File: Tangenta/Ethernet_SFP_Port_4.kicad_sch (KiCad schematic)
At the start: 17 parts, among them J9 HC-SFP-01L

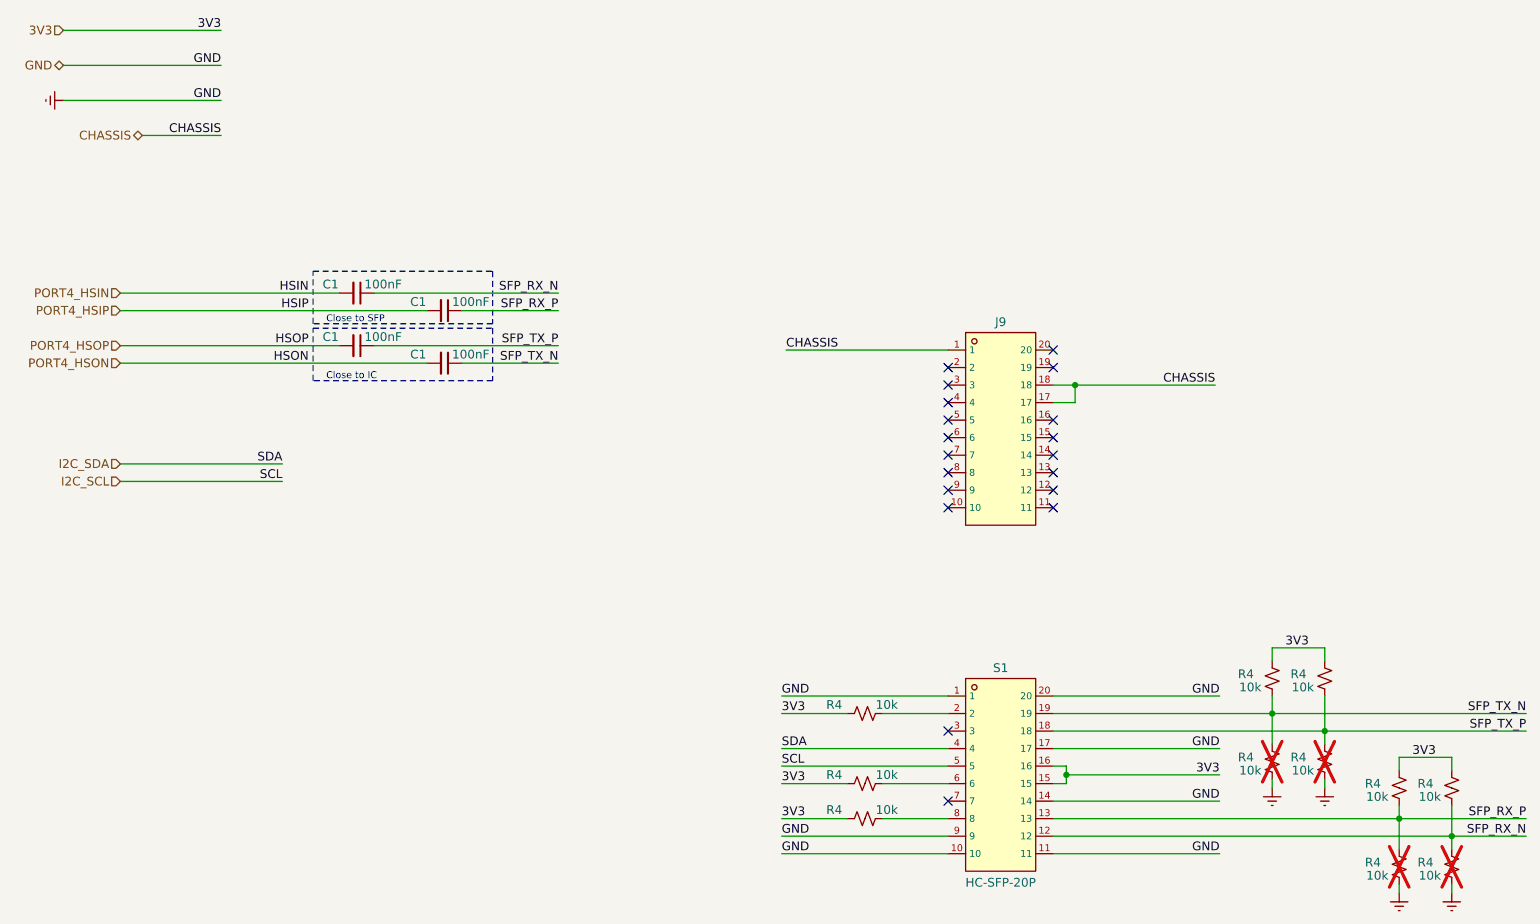
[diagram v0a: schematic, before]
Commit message: initialize branch
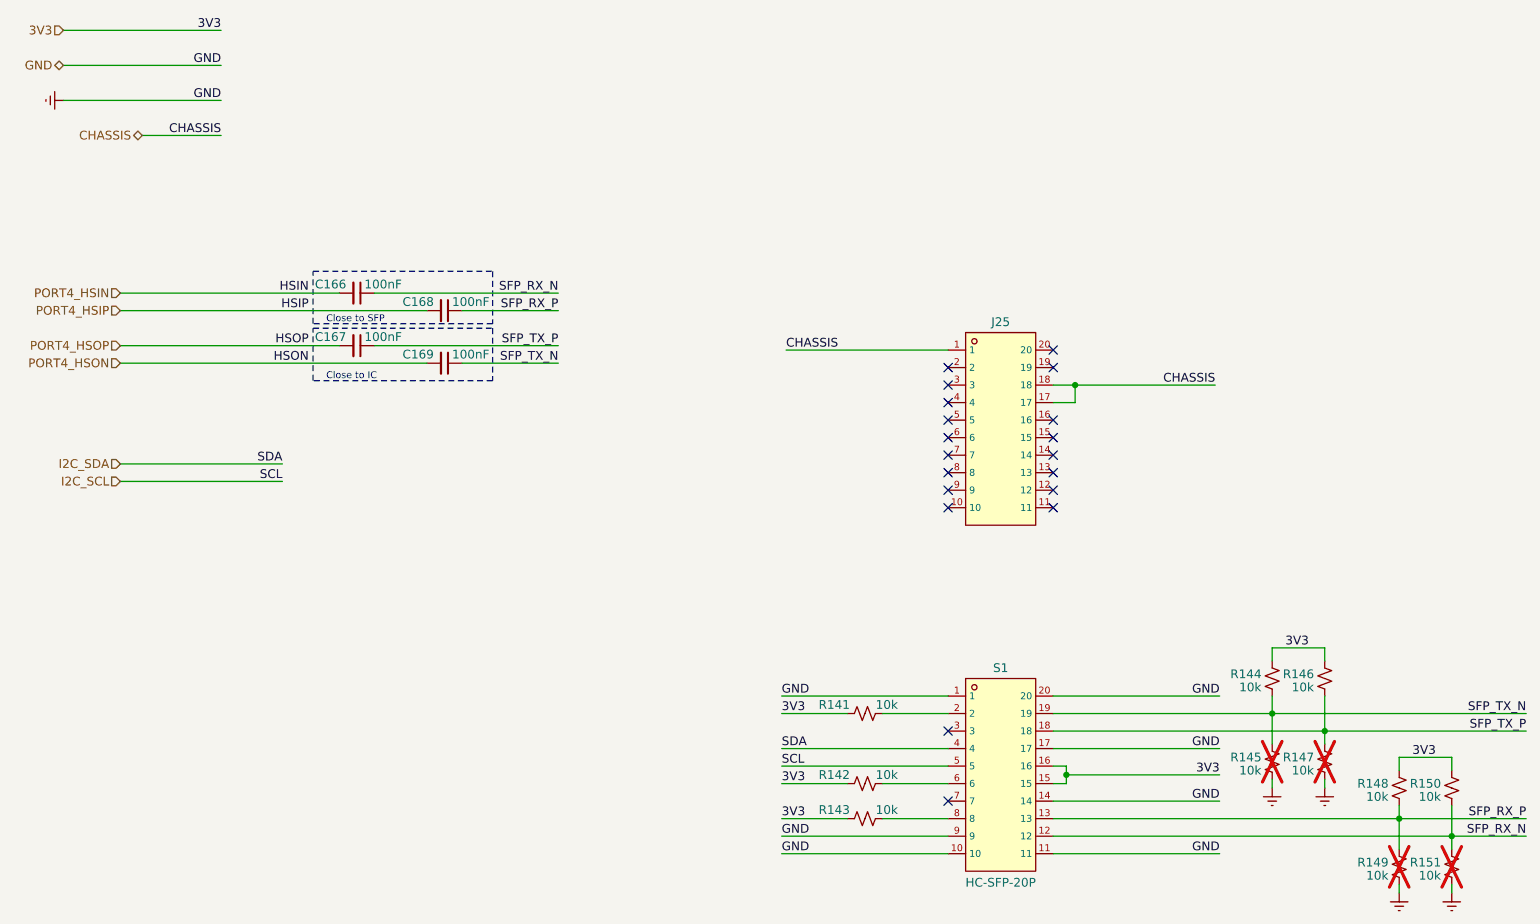
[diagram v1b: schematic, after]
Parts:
- renumbered C1 to C166, C1 to C167, C1 to C168, C1 to C169, J9 to J25, R4 to R141, R4 to R142, R4 to R143, R4 to R144, R4 to R145, R4 to R146, R4 to R147, R4 to R148, R4 to R149, R4 to R150, R4 to R151

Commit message: J6-J8,J22-J25,S1,U21
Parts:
- J25: footprint SFP_CAGE:TH_HC-SFP-01L -> CholaFootprintsPrjLib:TH_HC-SFP-01L
- S1: footprint SFP_Connector:SFP_Connector -> CholaFootprintsPrjLib:SFP_Connector
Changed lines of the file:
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@@
       (effects (font (size 1.27 1.27)) hide)
     )
-    (property "Footprint" "SFP_CAGE:TH_HC-SFP-01L" (at 159.385 86.995 0)
+    (property "Footprint" "CholaFootprintsPrjLib:TH_HC-SFP-01L" (at 159.385 86.995 0)
       (effects (font (size 1.27 1.27) italic) hide)
     )
@@
       (effects (font (size 1.27 1.27)))
     )
-    (property "Footprint" "SFP_Connector:SFP_Connector" (at 159.385 137.16 0)
+    (property "Footprint" "CholaFootprintsPrjLib:SFP_Connector" (at 159.385 137.16 0)
       (effects (font (size 1.27 1.27) italic) hide)
     )
